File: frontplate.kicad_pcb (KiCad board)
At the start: 2 copper layers, 200 x 105 mm, 5 parts

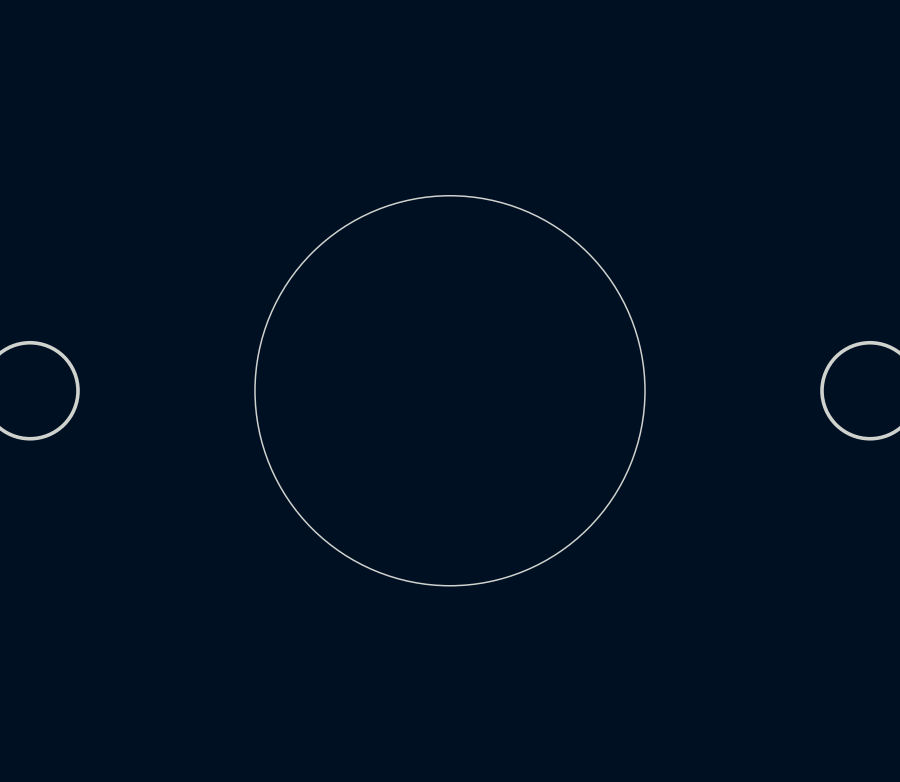
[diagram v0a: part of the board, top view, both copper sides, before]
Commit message: some cleaning
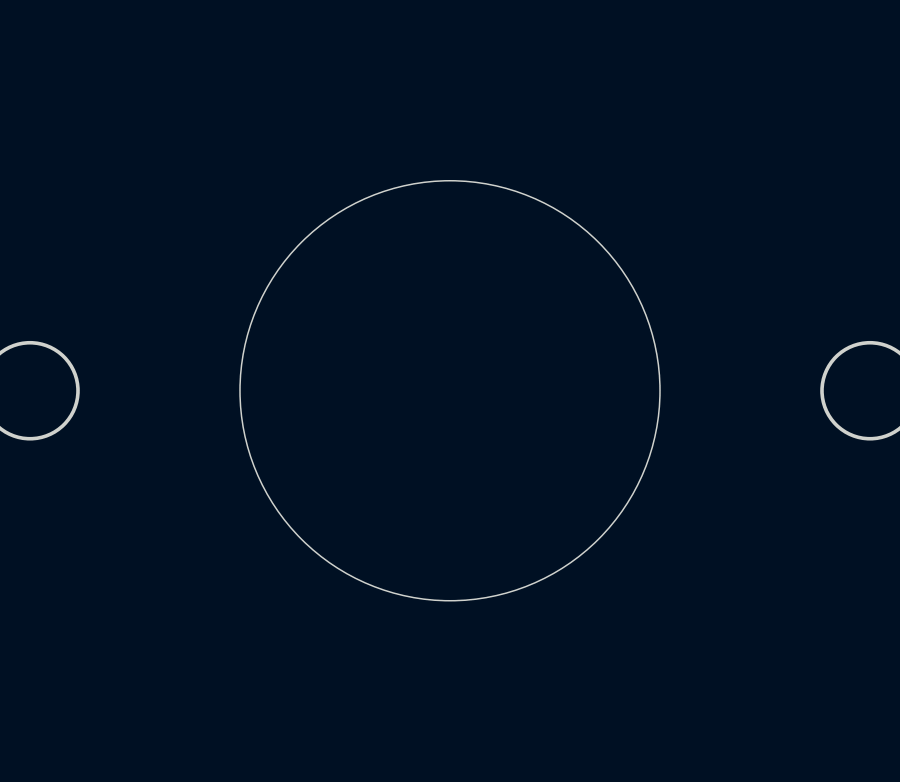
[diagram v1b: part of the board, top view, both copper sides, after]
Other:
- outline, holes or cut-outs redrawn
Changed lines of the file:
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@@
   (gr_circle (center 114.046 92.202) (end 115.796 92.202) (layer Edge.Cuts) (width 0.05))
   (gr_circle (center 114.173 102.489) (end 115.923 102.489) (layer Edge.Cuts) (width 0.05))
-  (gr_circle (center 139.008 123.413) (end 145.508 123.413) (layer Edge.Cuts) (width 0.05))
+  (gr_circle (center 139.008 123.413) (end 146.008 123.413) (layer Edge.Cuts) (width 0.05))
   (gr_line (start 38.933 45.208) (end 238.933 45.208) (layer Edge.Cuts) (width 0.05))
   (gr_text "200mm x 105mm" (at 57.531 160.147) (layer Eco2.User)
